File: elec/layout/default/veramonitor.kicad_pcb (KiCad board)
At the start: 2 copper layers, 111.2 x 70.4 mm, 98 parts, among them J1 ?, U1 ?, U10 ?, U11 ?, U12 ?, U13 ?, U14 ?, U15 ?, U16 ?, U17 ?, U18 ?, U19 ?, U2 ?, U20 ?, U21 ?, U22 ?, U23 ?, U24 ?, U25 ?, U26 ?, U27 ?, U28 ?, U29 ?, U3 ?, U30 ?, U31 ?, U32 ?, U33 ?, U34 ?, U35 ?, U36 ?, U37 ?, U38 ?, U39 ?, U4 ?, U40 ?, U41 ?, U42 ?, U43 ?, U44 ?, U45 ?, U46 ?, U47 ?, U48 ?, U5 ?, U6 ?, U7 ?, U8 ?, U9 ?

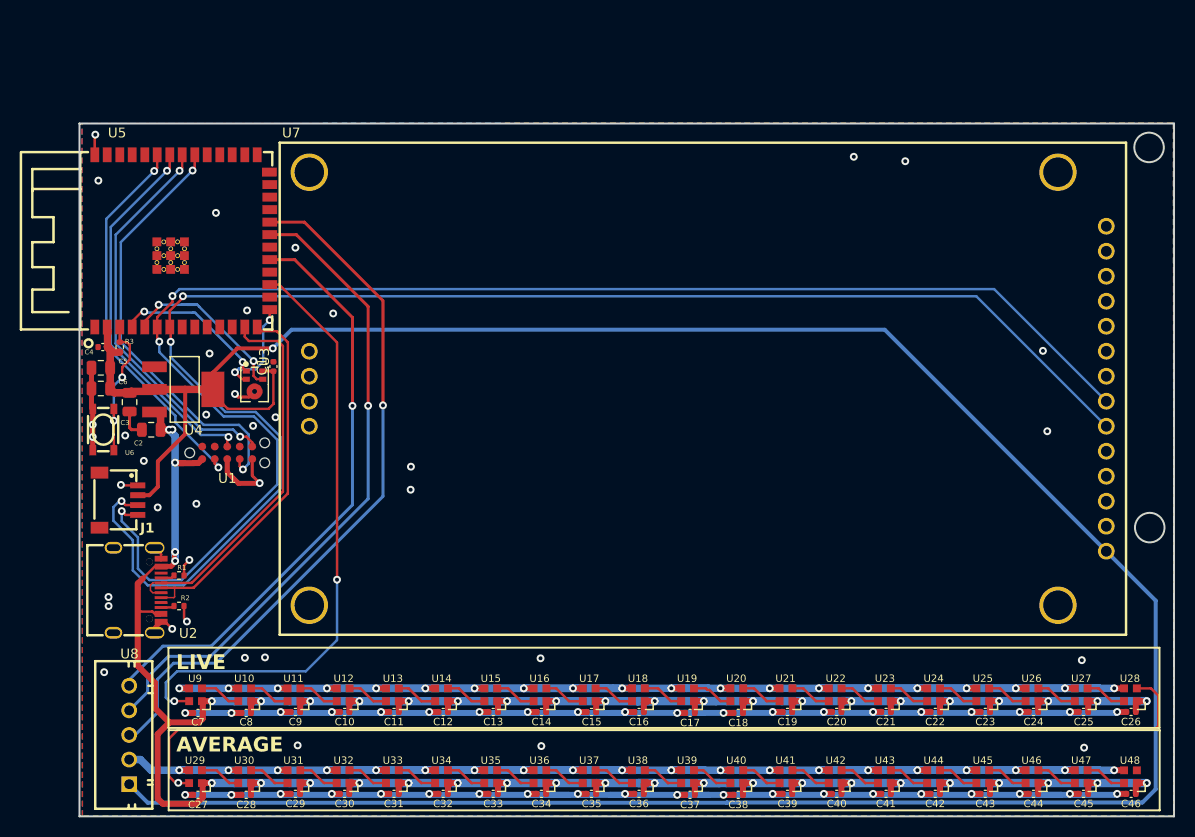
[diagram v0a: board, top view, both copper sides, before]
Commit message: edits
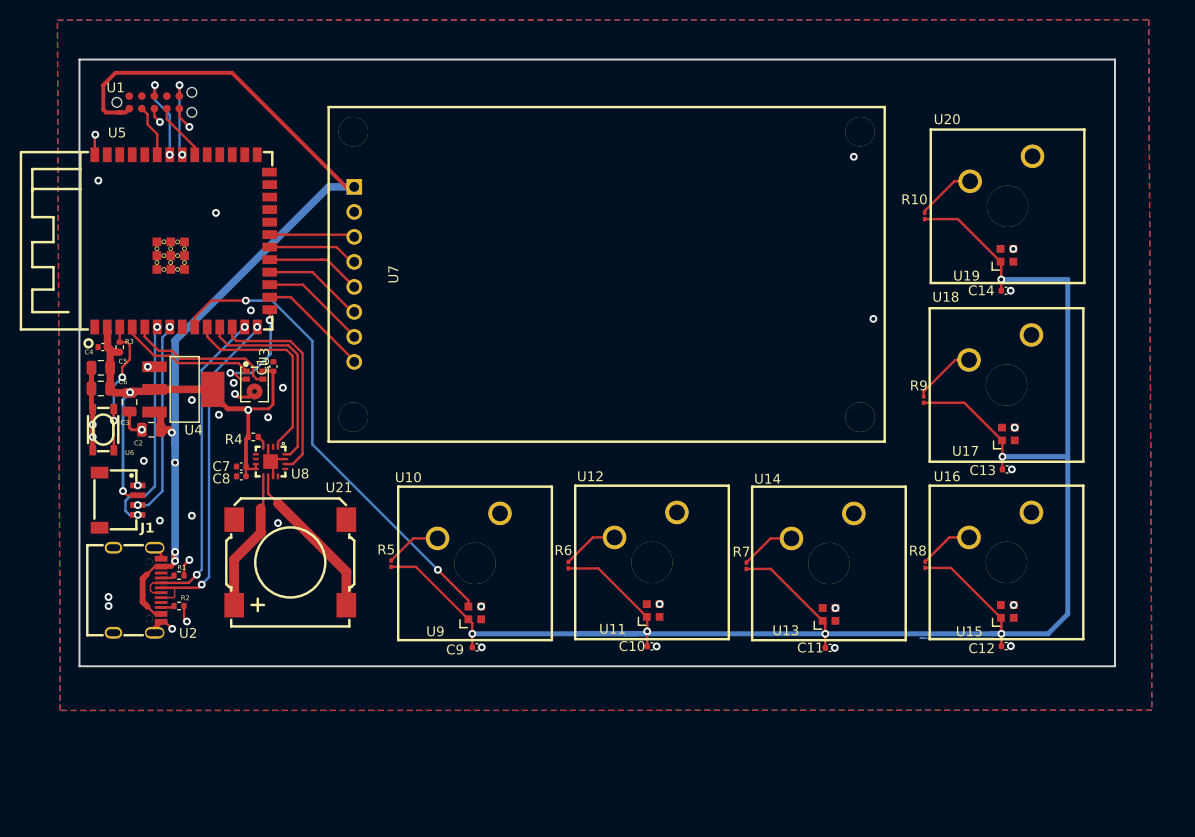
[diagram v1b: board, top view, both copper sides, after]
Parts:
- removed C15, C16, C17, C18, C19, C20, C21, C22, C23, C24, C25, C26, C27, C28, C29, C30, C31, C32, C33, C34, C35, C36, C37, C38, C39, C40, C41, C42, C43, C44, C45, C46: 16V 100nF X7R ±10% 0402 Multilayer Ceramic Capacitors MLCC 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, lib:C0402
- removed U22, U23, U24, U25, U26, U27, U28, U29, U30, U31, U32, U33, U34, U35, U36, U37, U38, U39, U40, U41, U42, U43, U44, U45, U46, U47, U48: ?, lib:LED-SMD_4P-L2.0-W2.0-BR
- added R10: 50mW Thick Film Resistors 25V ±1% ±200ppm/℃ 10kΩ 0201 Chip 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, lib:R0201, F.Cu at (126.0, 76.3)
- added R4: 62.5mW Thick Film Resistors 50V ±100ppm/℃ ±1% 10kΩ 0402 Chi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, lib:R0402, F.Cu at (57.7, 98.8)
- added R5: 50mW Thick Film Resistors 25V ±1% ±200ppm/℃ 10kΩ 0201 Chip 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, lib:R0201, F.Cu at (71.7, 111.6)
- added R6: 50mW Thick Film Resistors 25V ±1% ±200ppm/℃ 10kΩ 0201 Chip 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, lib:R0201, F.Cu at (89.7, 111.8)
- added R7: 50mW Thick Film Resistors 25V ±1% ±200ppm/℃ 10kΩ 0201 Chip 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, lib:R0201, F.Cu at (107.8, 111.8)
- added R8: 50mW Thick Film Resistors 25V ±1% ±200ppm/℃ 10kΩ 0201 Chip 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, lib:R0201, F.Cu at (126.0, 111.7)
- added R9: 50mW Thick Film Resistors 25V ±1% ±200ppm/℃ 10kΩ 0201 Chip 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, lib:R0201, F.Cu at (125.9, 95.0)
- C7: value 16V 100nF X7R ±10% 0402 Multilayer Ceramic Capacitors MLCC - SMD/SMT ROHS -> 6.3V 10uF X5R ±20% 0402 Multilayer Ceramic Capacitors MLCC - SMD/SMT ROHS
- U10, U12, U14, U16, U18, U20: footprint lib:LED-SMD_4P-L2.0-W2.0-BR -> lib:KEY-TH_CPG1511F01S0X
- U21: footprint lib:LED-SMD_4P-L2.0-W2.0-BR -> lib:BUZ-SMD_4P-L13.0-W13.0-P11.4-BL
- U7: footprint lib:COMM-TH_HS12864G18B -> lib:LCD-TH_L56.5-W34.0_1-8INCH-LCD-MODULE
- U8: footprint lib:CONN-TH_5P-P2.50_XH-5A_C2318 -> lib:TQFN-16_L3.0-W3.0-P0.50-BL-EP1.5
- moved C14 63.7 mm to (134.2, 83.9), turned to 0 degrees
- moved U20 59.8 mm to (133.8, 71.5)
- moved C13 57.7 mm to (134.3, 102.0), turned to 0 degrees
- moved C12 57.6 mm to (134.2, 120.0), turned to 0 degrees
- moved U19 55.2 mm to (134.3, 80.3), turned to -90 degrees
- moved U15 53.2 mm to (134.4, 116.5), turned to -90 degrees
- moved U21 52.1 mm to (61.5, 111.5)
- moved U18 51.0 mm to (133.6, 89.7)
- moved U17 50.2 mm to (134.5, 98.4), turned to -90 degrees
- moved U16 49.8 mm to (133.6, 107.7)
- moved U13 45.1 mm to (116.2, 116.8), turned to -90 degrees
- moved C11 44.8 mm to (116.3, 120.2), turned to 0 degrees
- moved U14 42.4 mm to (115.6, 107.8)
- moved U7 37.8 mm to (68.0, 82.2), turned to -90 degrees
- moved U11 37.5 mm to (98.4, 116.4), turned to -90 degrees
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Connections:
- net reset renamed jtag_connector-reset
- C10 pad 1: vcc -> vcc-1
- C11 pad 1: vcc -> vcc-1
- C12 pad 1: vcc -> vcc-1
- C13 pad 1: vcc -> vcc-1
- C14 pad 1: vcc -> vcc-1
- C7 pad 1: vcc -> vcc-1
- C8 pad 1: vcc -> vcc-1
- C9 pad 1: vcc -> vcc-1
- U10 pad 1: vcc -> sw1-key
- U10 pad 2: ledrow1.led2.ic-vcc -> gnd
- U11 pad 1: vcc -> vcc-1
- U11 pad 2: ledrow1.led3.ic-vcc -> sw2-dout
- U11 pad 4: ledrow1.led2.ic-vcc -> sw1-dout
- U12 pad 1: vcc -> sw2-key
- U12 pad 2: ledrow1.led4.ic-vcc -> gnd
- U13 pad 1: vcc -> vcc-1
- U13 pad 2: ledrow1.led5.ic-vcc -> sw3-dout
- U13 pad 4: ledrow1.led4.ic-vcc -> sw2-dout
- U14 pad 1: vcc -> sw3-key
- U14 pad 2: ledrow1.led6.ic-vcc -> gnd
- U15 pad 1: vcc -> vcc-1
- U15 pad 2: ledrow1.led7.ic-vcc -> sw4-dout
- U15 pad 4: ledrow1.led6.ic-vcc -> sw3-dout
- U16 pad 1: vcc -> sw4-key
- U16 pad 2: ledrow1.led8.ic-vcc -> gnd
- U17 pad 1: vcc -> vcc-1
- U17 pad 2: ledrow1.led9.ic-vcc -> sw5-dout
- U17 pad 4: ledrow1.led8.ic-vcc -> sw4-dout
- U18 pad 1: vcc -> sw5-key
- U18 pad 2: ledrow1-dout -> gnd
- U19 pad 1: vcc -> vcc-1
- U19 pad 2: ledrow2.led1.ic-vcc -> sw6-dout
- U19 pad 4: ledrow1-dout -> sw5-dout
- U20 pad 1: vcc -> sw6-key
- U20 pad 2: ledrow2.led2.ic-vcc -> gnd
- U21 pad 1: vcc -> outp
- U21 pad 2: ledrow2.led3.ic-vcc -> outn
- U21 pad 3: gnd -> dummy
- U21 pad 4: ledrow2.led2.ic-vcc -> dummy
- U5 pad 10: io17 -> din
- U5 pad 11: io18 -> bclk
- U5 pad 12: io8 -> lrclk
- U5 pad 16: io46 -> backlighten
- U5 pad 17: led_data -> micro.ic-reset
- U5 pad 18: io10 -> dc
- U5 pad 19: p5 -> cs
- U5 pad 20: io12 -> sck
- U5 pad 21: p4 -> mosi
- U5 pad 22: p3 -> io14
- U7 pad 1: vcc-1 -> vcc
- U7 pad 3: cs -> mosi
- U7 pad 4: rst -> sck
- U7 pad 5: a0 -> cs
- U7 pad 6: sda -> dc
- U7 pad 7: scl -> micro.ic-reset
- U7 pad 8: led -> backlighten
- U8 pad 1: vcc-1 -> din
- U8 pad 2: gnd -> gain_slot
- U8 pad 3: p3 -> gnd
- U8 pad 4: p4 -> sd_mode_hash
- U8 pad 5: p5 -> n_period_c_period
- U9 pad 1: vcc -> vcc-1
- U9 pad 2: ledrow1.led1.ic-vcc -> sw1-dout
- U9 pad 4: led_data -> io16
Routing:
- net gnd: track 680.5 -> 36.0 mm, vias 117 -> 39
- net vcc: track 386.7 -> 103.0 mm, vias 45 -> 4
- net sda: track 155.8 -> 20.2 mm, vias 3 -> 2
- net scl: track 153.5 -> 22.3 mm, vias 3 -> 2
- net ledrow2-dout: track 112.8 -> 0.00 mm, vias 1 -> 0
- net p3: track 72.5 -> 0.00 mm, vias 1 -> 0
- net p4: track 66.6 -> 0.00 mm, vias 1 -> 0
- net led_data: track 62.7 -> 0.00 mm, vias 2 -> 0
- net p5: track 60.5 -> 0.00 mm, vias 1 -> 0
- net io16: track 0.00 -> 48.9 mm, vias 0 -> 2
- net tck: track 44.0 -> 5.86 mm, vias 2 -> 0
- net tms: track 39.9 -> 5.34 mm, vias 2 -> 0
- net tdo: track 40.4 -> 8.31 mm
- net tdi: track 38.8 -> 8.84 mm
- net lrclk: track 0.00 -> 21.3 mm
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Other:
- board size 111.2 x 70.4 mm -> 105.2 x 61.6 mm
- board text removed: "AVERAGE"
- board text removed: "LIVE"
